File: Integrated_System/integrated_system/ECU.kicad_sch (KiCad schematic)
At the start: 8 parts, among them J1 Jack-DC, U2 IRLR7843, U3 IRLR7843, U4 IRLR7843

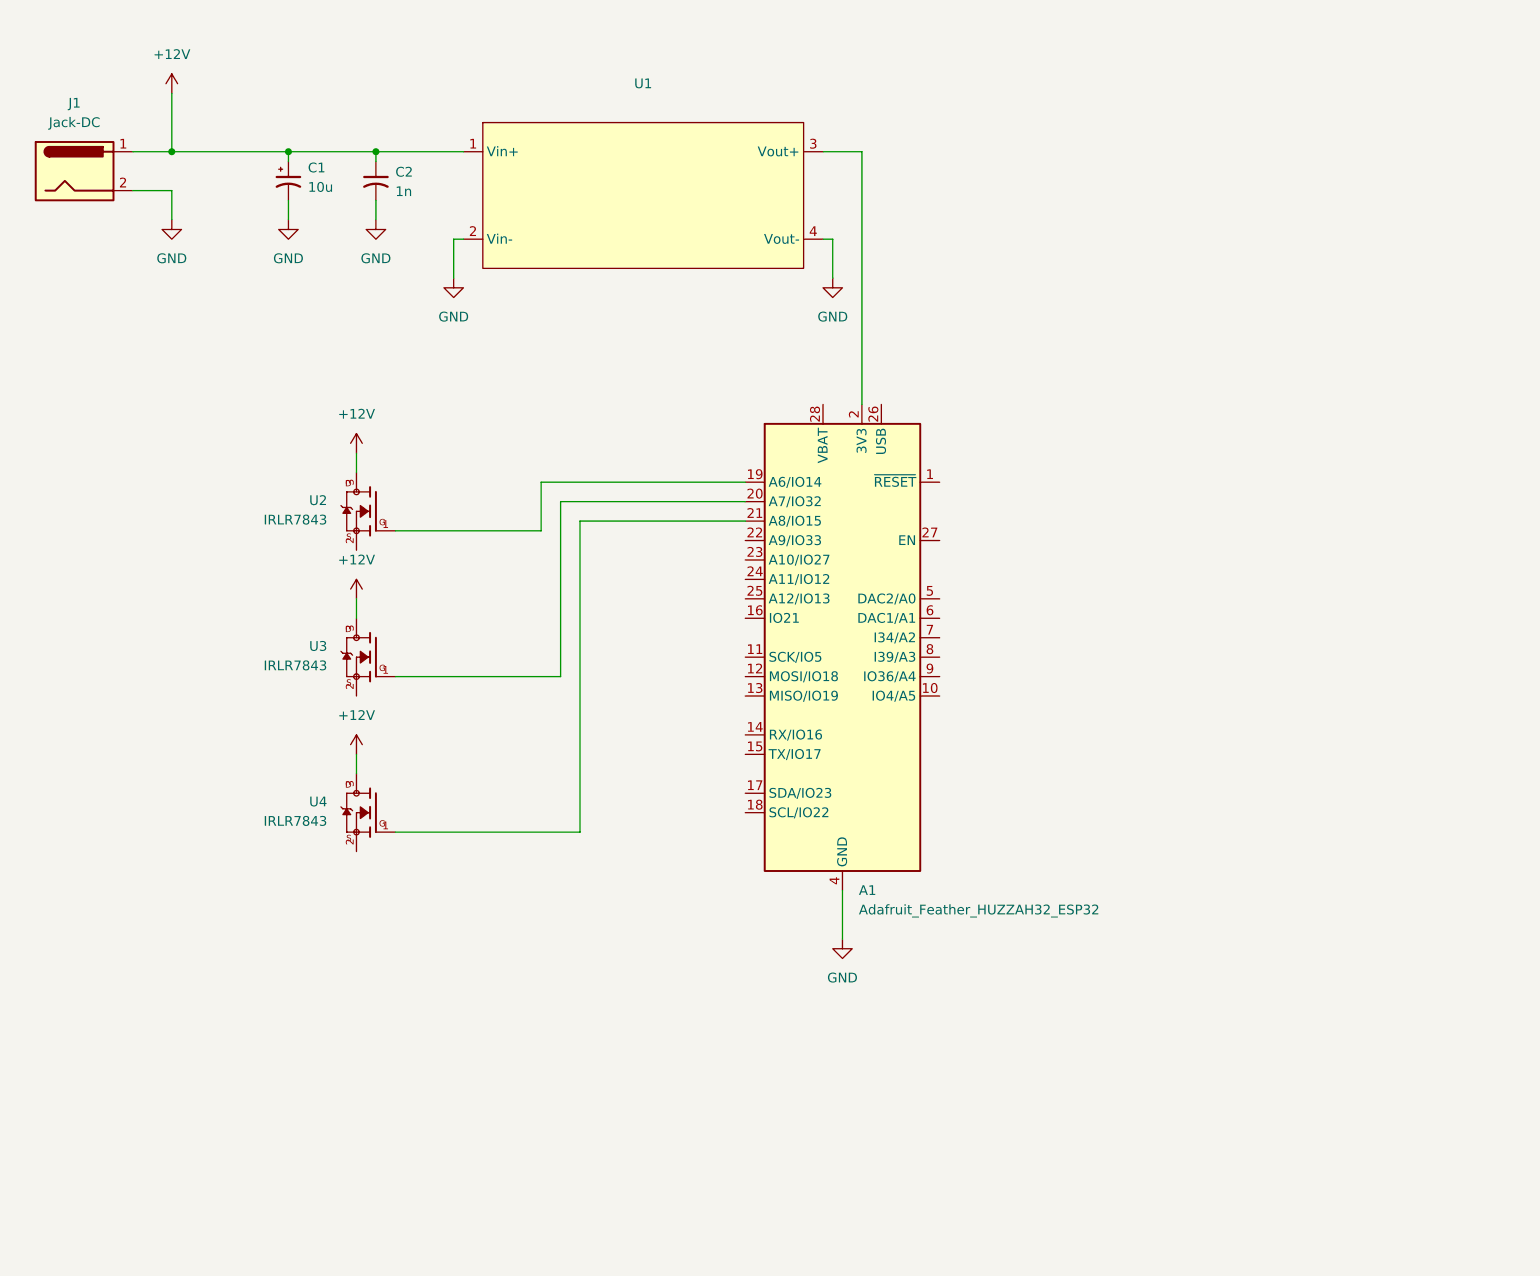
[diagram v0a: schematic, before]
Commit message: Added Sensors
Made a bunch of changes
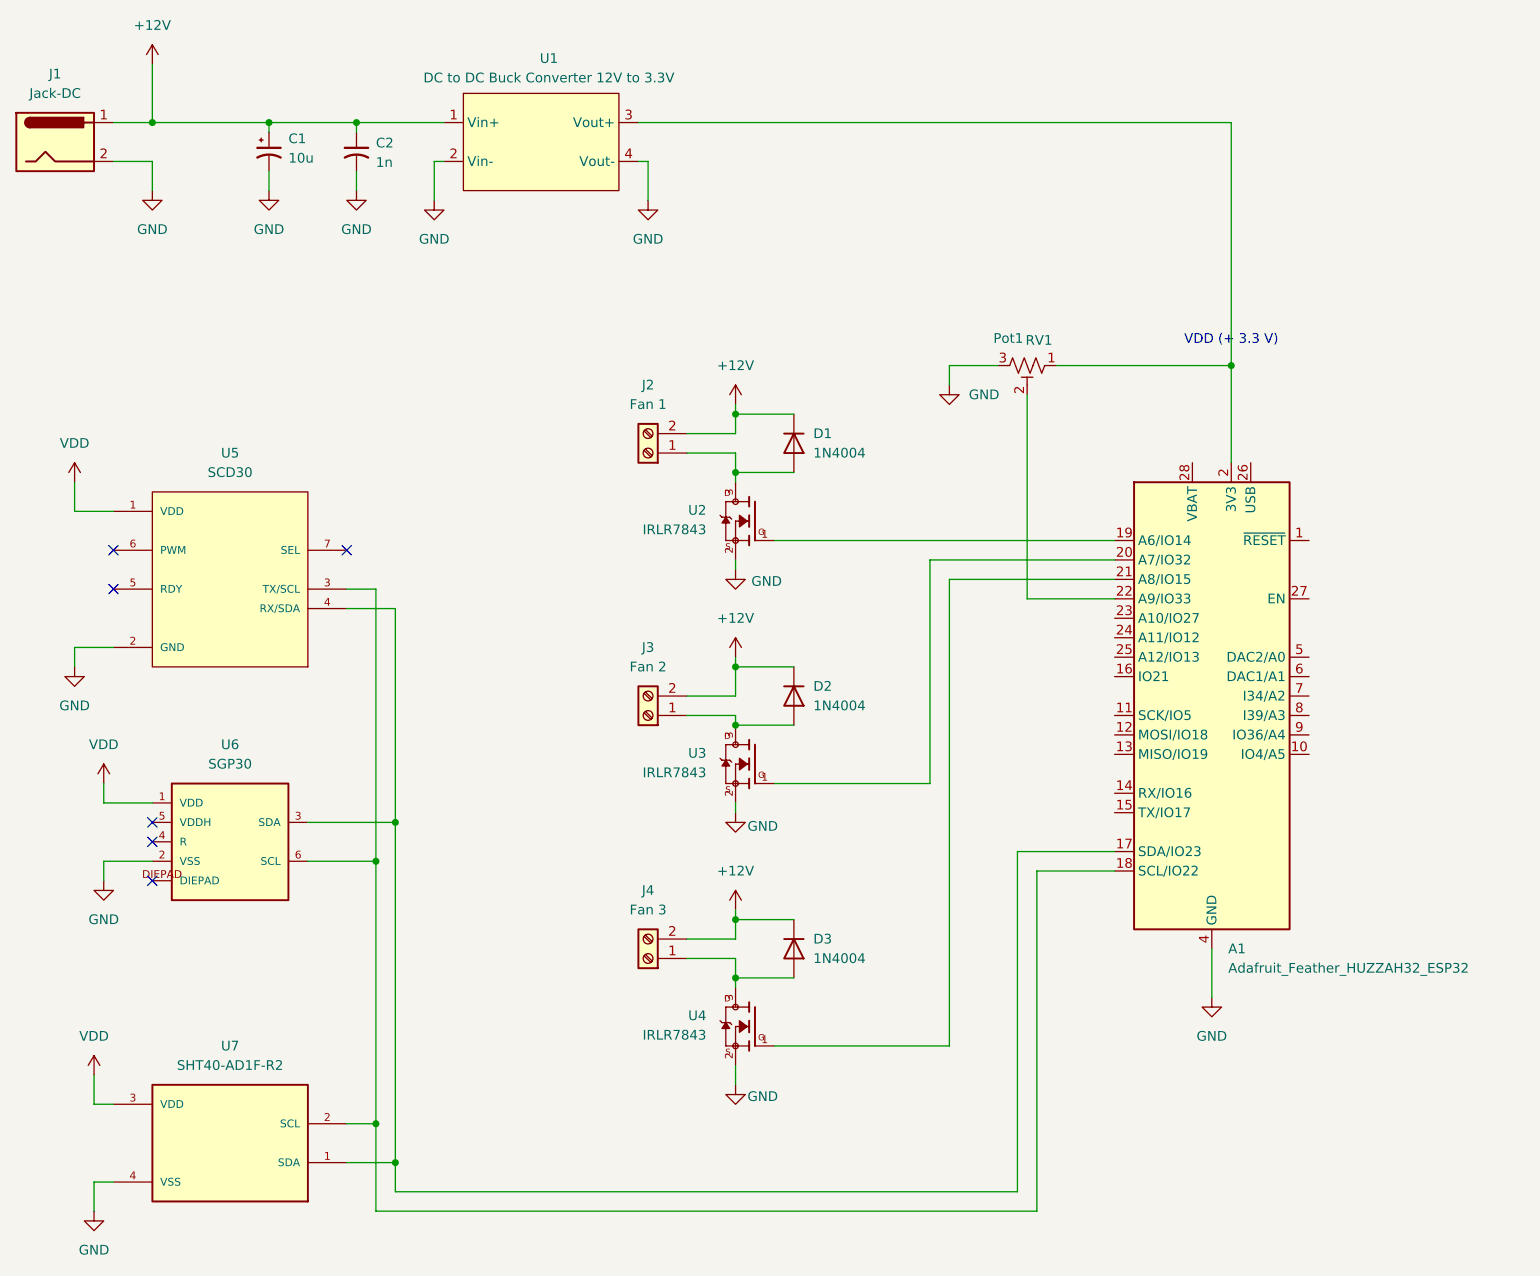
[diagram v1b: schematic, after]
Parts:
- added D1, D2, D3: 1N4004, Diode_THT:D_DO-41_SOD81_P10.16mm_Horizontal, symbol Diode:1N4004
- added J2: Fan 1, symbol Connector:Screw_Terminal_01x02
- added J3: Fan 2, symbol Connector:Screw_Terminal_01x02
- added J4: Fan 3, symbol Connector:Screw_Terminal_01x02
- added RV1: Pot1, symbol Device:R_Potentiometer_Trim_US
- added U5: SCD30, SCD30:MODULE_SCD30, symbol SCD30:SCD30
- added U6: SGP30, SGP30:SGP30, symbol SGP30:SGP30
- added U7: SHT40-AD1F-R2, SHT40-AD1F-R2:SHT4X, symbol SHT40-AD1F-R2:SHT40-AD1F-R2
- U1: value ~ -> DC to DC Buck Converter 12V to 3.3V
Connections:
- net +12V: now also D1.1 (K), D2.1 (K), D3.1 (K), J2.2 (Pin_2), J3.2 (Pin_2), J4.2 (Pin_2); no longer U2.3, U3.3, U4.3
- net GND: now also U2.2, U3.2, U4.2, RV1.3, U5.2 (GND), U6.2 (VSS), U7.4 (VSS)
- net at A1.17 (SDA/IO23): now also U5.4 (RX/SDA), U6.3 (SDA), U7.1 (SDA)
- net at A1.18 (SCL/IO22): now also U5.3 (TX/SCL), U6.6 (SCL), U7.2 (SCL)
- net at A1.2 (3V3), U1.3 (Vout+): now also RV1.1
- net at A1.22 (A9/IO33): now also RV1.2
- new net: D3.2 (A), J4.1 (Pin_1), U4.3
- new net: D1.2 (A), J2.1 (Pin_1), U2.3
- new net: D2.2 (A), J3.1 (Pin_1), U3.3
- new net VDD: U5.1 (VDD), U6.1 (VDD), U7.3 (VDD)
- no-connect marks 0 -> 6
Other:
- note added: "VDD (+ 3.3 V)"
- moved on the sheet: A1, C1, C2, J1, U1, U2, U3, U4
